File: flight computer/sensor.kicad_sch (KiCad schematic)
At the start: 112 parts, among them IC1 A3909, J1 Micro_SD_Card_Det1, J12 Conn_01x04, J13 1x3 servo, J14 1x3 servo, J15 arming terminal, J16 arming terminal, J17 H9161TR-ND, J19 Screw_Terminal_01x02, J20 Screw_Terminal_01x02, J3 H9161TR-ND, J4 H9161TR-ND, J5 Screw_Term, J6 1x3 servo, J9 1x3 servo, Q1 IRLML6402, Q3 IRLML6402, Q4 IRLML6402, Q5 IRLML6402, Q6 IRLML6402, Q7 BSS138, Q8 IRLML6402, Q9 IRLML6402, U10 LSM6DS3, U11 BGM220SC12WGA2R, U16 SX1262IMLTRT, U17 PE4259, U5 LPS22HB, U6 GPS, U8 NAND, Y2 32MHz

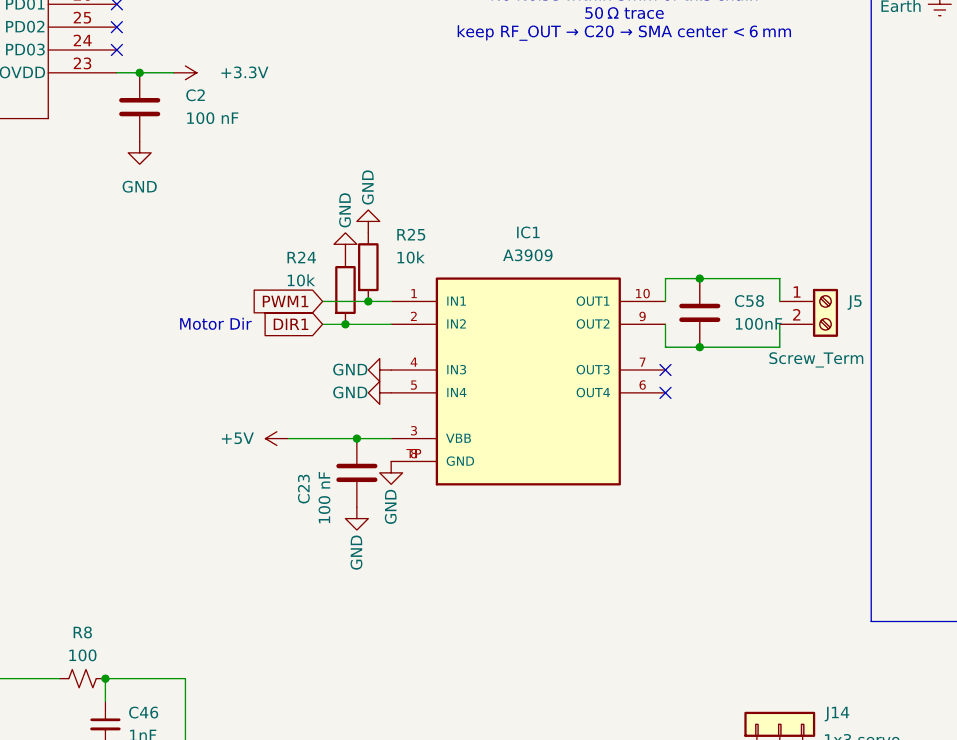
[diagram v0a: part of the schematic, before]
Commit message: more wiring kms
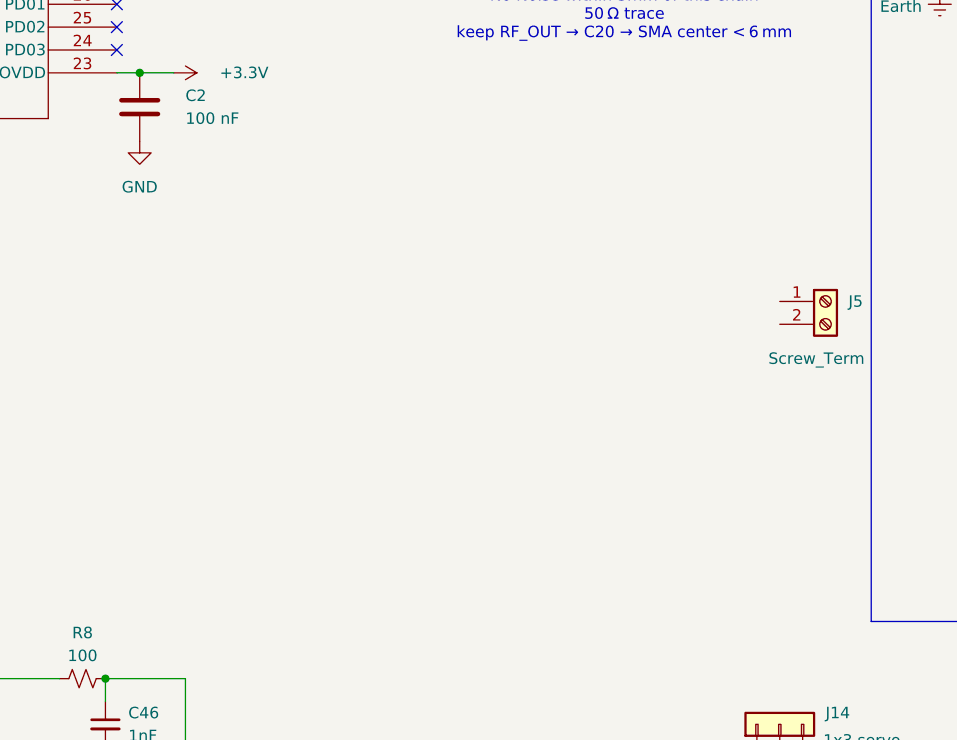
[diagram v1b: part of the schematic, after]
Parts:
- removed C23: 100 nF, Capacitor_SMD:C_0603_1608Metric, symbol Device:C
- removed C58: 100nF, Capacitor_SMD:C_0603_1608Metric, symbol Device:C
- removed IC1: A3909, A3909:MSOP10-PAD, symbol A3909:A3909
- removed R24, R25: 10k, Resistor_SMD:R_0603_1608Metric, symbol Device:R
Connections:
- no-connect marks 41 -> 39
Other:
- note removed: "Motor Dir"

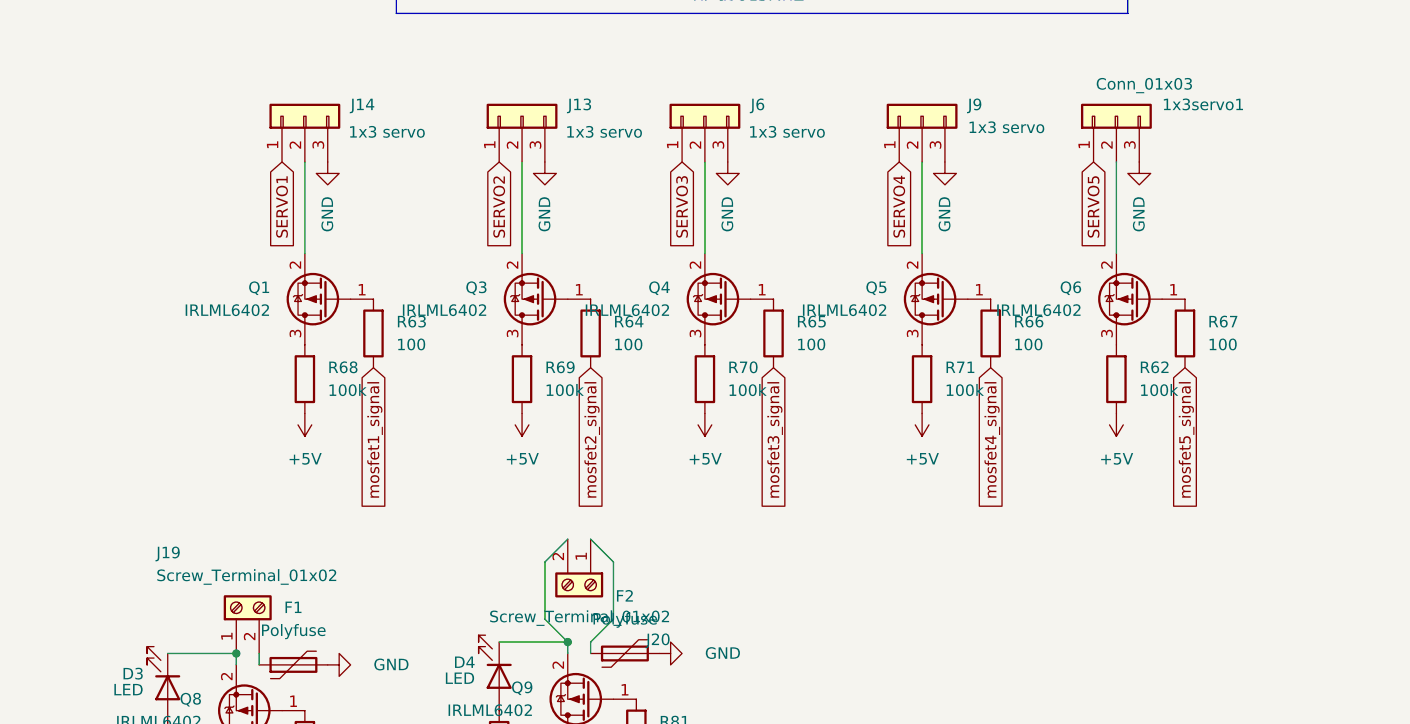
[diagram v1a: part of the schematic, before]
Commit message: wiring fml
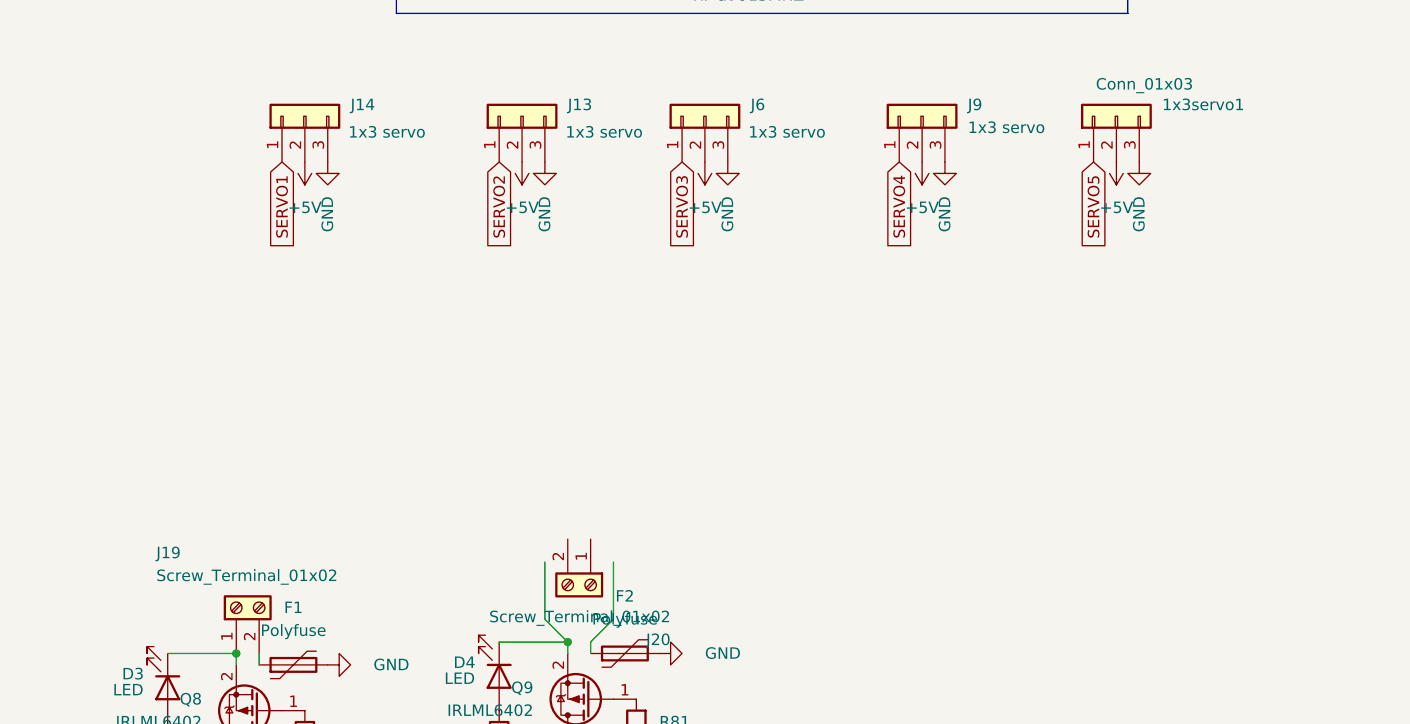
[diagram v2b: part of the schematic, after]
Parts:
- removed Q1, Q3, Q4, Q5, Q6: IRLML6402, Package_TO_SOT_SMD:SOT-23, symbol Transistor_FET:IRLML6402
- removed R62, R68, R69, R70, R71: 100k, Resistor_SMD:R_0603_1608Metric, symbol Device:R
- removed R63, R64, R65, R66, R67: 100, Resistor_SMD:R_0603_1608Metric, symbol Device:R
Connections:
- net +5V: now also 1x3servo1.2 (Pin_2), J13.2 (Pin_2), J14.2 (Pin_2), J6.2 (Pin_2), J9.2 (Pin_2)
- net at D4.1 (K), Q9.2 (S): no longer J20.2 (Pin_2)
- net at J20.1 (Pin_1): no longer F2.1
